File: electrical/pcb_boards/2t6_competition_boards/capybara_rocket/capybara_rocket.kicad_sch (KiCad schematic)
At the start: 110 parts, among them J1 3.6V Battery, J10 Elevator, J11 SparkFun MAX-M10S, J12 Aileron 1, J13 Aileron 2, J14 Ground Camera, J15 Payload Camera, J16 DC Motor, J2 1.2V Battery, J3 3.6V Switch, J4 1.2V Switch, J5 LED, J6 NC, J7 CC, J8 VL53L1-SATEL, J9 Egg, Q1 SI4435DDY, Q2 SI4435DDY, U1 DS1307+, U10 TPS3839, U11 MP3414, U12 SN74LVC1G04, U13 MCP1640, U14 TPS3839, U15 STM32 NUCLEO-G431KB, U16 SN74AUP1G04, U17 SparkFun XBee Explorer, U2 Adafruit BNO085, U3 TLC555, U4 EEPROM, U5 LTC3536, U6 LTC3536, U7 Adafruit BMP581, U8 DRV8212, U9 INA219, Y1 AB38T-32.768KHZ

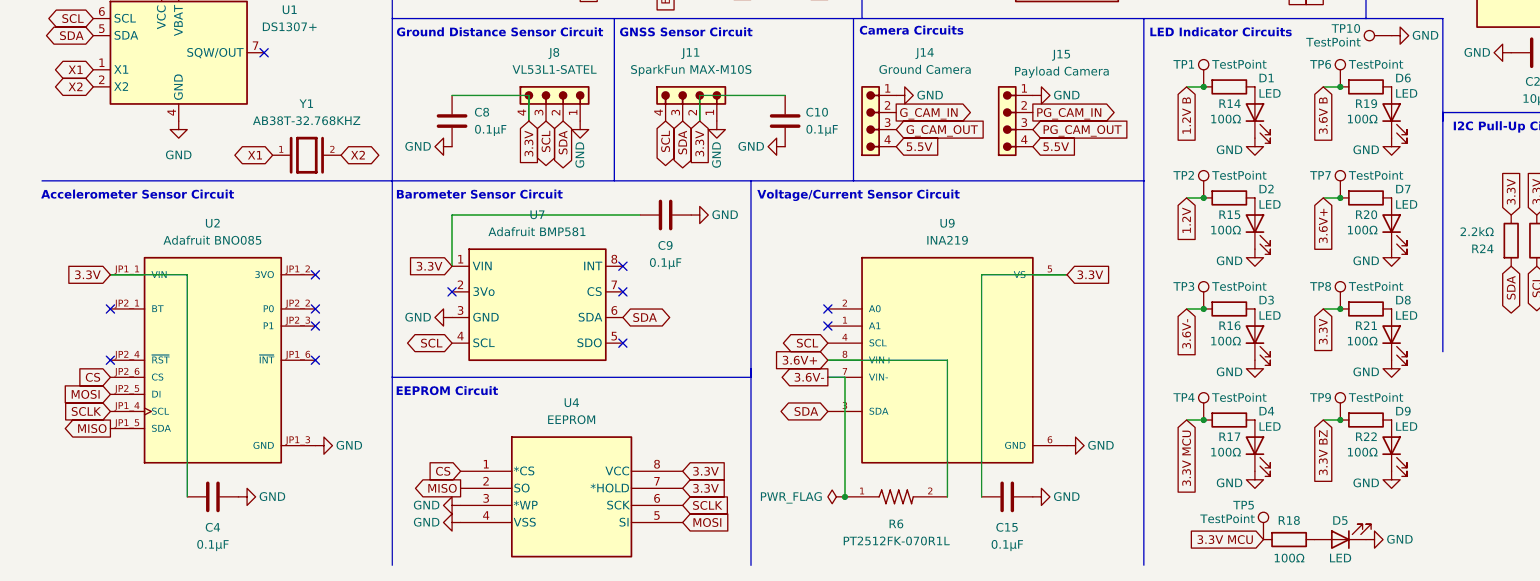
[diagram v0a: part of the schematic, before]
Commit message: New graphics and layout work
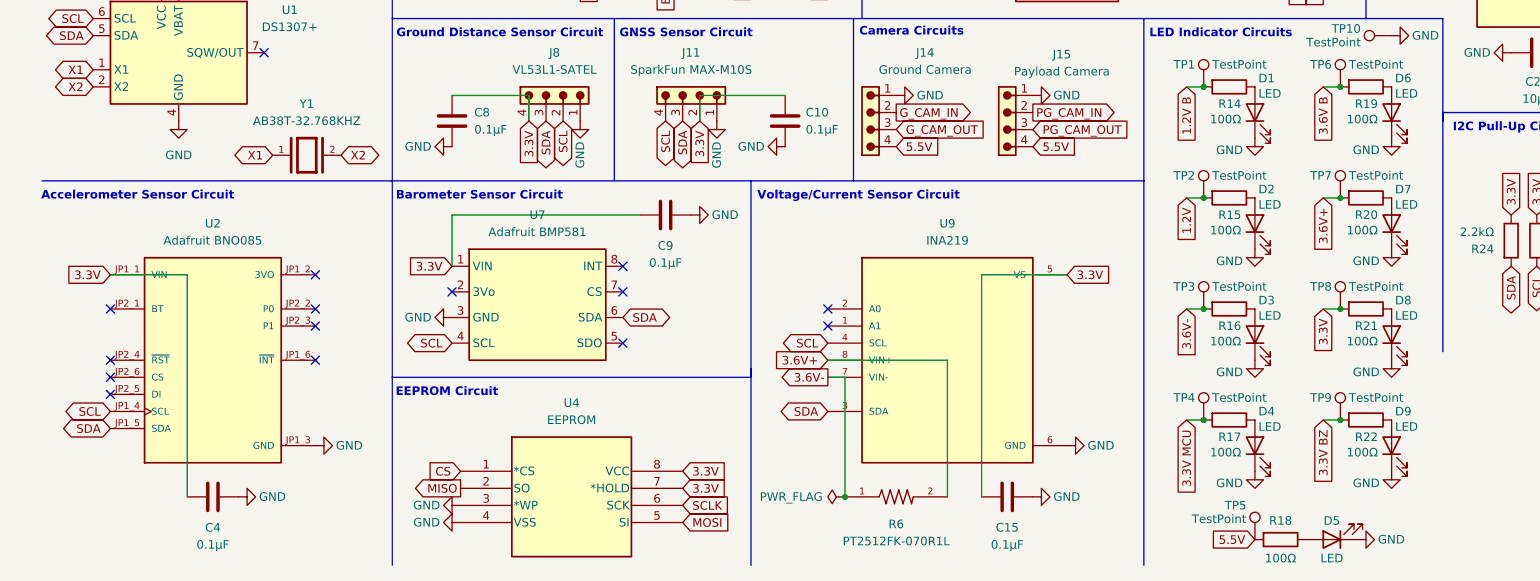
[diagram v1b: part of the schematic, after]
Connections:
- net 3.3V MCU: no longer R18.2, TP5.1
- net 5.5V: now also R18.2, TP5.1
- net CS: no longer U2.JP2_6 (CS)
- net MISO: no longer U2.JP1_5 (SDA)
- net MOSI: no longer U2.JP2_5 (DI)
- net SCL: now also J8.2, U2.JP1_4 (SCL); no longer J8.3
- net SCLK: no longer U2.JP1_4 (SCL)
- net SDA: now also J8.3, U2.JP1_5 (SDA); no longer J8.2
- no-connect marks 62 -> 64
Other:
- moved on the sheet: D5, R18, TP5
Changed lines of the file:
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@@
 	)
 	(no_connect
+		(at 22.86 171.45)
+	)
+	(no_connect
 		(at 29.21 71.12)
 	)
@@
 	)
 	(no_connect
+		(at 22.86 168.91)
+	)
+	(no_connect
 		(at 99.06 152.4)
 	)
@@
 		)
 	)
-	(global_label "MOSI"
-		(shape input)
-		(at 22.86 171.45 180)
-		(fields_autoplaced yes)
-		(effects
-			(font
-				(size 1.27 1.27)
-			)
-			(justify right)
-		)
-		(property "Intersheetrefs" "${INTERSHEET_REFS}"
-			(at 15.2786 171.45 0)
-			(effects
-				(font
-					(size 1.27 1.27)
-				)
-				(justify right)
-				(hide yes)
-			)
-		)
-	)
 	(global_label "SDA"
 		(shape bidirectional)
@@
 		)
 	)
-	(global_label "3.3V MCU"
+	(global_label "5.5V"
 		(shape input)
-		(at 194.31 193.04 180)
+		(at 193.04 193.04 180)
 		(fields_autoplaced yes)
 		(effects
@@
 		)
 		(property "Intersheetrefs" "${INTERSHEET_REFS}"
-			(at 182.1929 193.04 0)
+			(at 185.9424 193.04 0)
 			(effects
 				(font
@@
 		)
 	)
+	(global_label "SCL"
+		(shape bidirectional)
+		(at 90.17 130.81 270)
+		(fields_autoplaced yes)
+		(effects
+			(font
+				(size 1.27 1.27)
+			)
+			(justify right)
+		)
+		(property "Intersheetrefs" "${INTERSHEET_REFS}"
+			(at 90.17 138.4141 90)
+			(effects
+				(font
+					(size 1.27 1.27)
+				)
+				(justify right)
+				(hide yes)
+			)
+		)
+	)
 	(global_label "SDA"
 		(shape bidirectional)
@@
 		)
 	)
-	(global_label "SDA"
-		(shape bidirectional)
-		(at 90.17 130.81 270)
-		(fields_autoplaced yes)
-		(effects
-			(font
-				(size 1.27 1.27)
-			)
-			(justify right)
-		)
-		(property "Intersheetrefs" "${INTERSHEET_REFS}"
-			(at 90.17 138.4746 90)
-			(effects
-				(font
-					(size 1.27 1.27)
-				)
-				(justify right)
-				(hide yes)
-			)
-		)
-	)
 	(global_label "NC_REL"
 		(shape output)
@@
 		)
 	)
-	(global_label "CS"
-		(shape input)
-		(at 22.86 168.91 180)
-		(fields_autoplaced yes)
-		(effects
-			(font
-				(size 1.27 1.27)
-			)
-			(justify right)
-		)
-		(property "Intersheetrefs" "${INTERSHEET_REFS}"
-			(at 17.3953 168.91 0)
-			(effects
-				(font
-					(size 1.27 1.27)
-				)
-				(justify right)
-				(hide yes)
-			)
-		)
-	)
 	(global_label "AILERON"
 		(shape input)
@@
 		)
 	)
-	(global_label "MISO"
-		(shape output)
-		(at 22.86 176.53 180)
-		(fields_autoplaced yes)
-		(effects
-			(font
-				(size 1.27 1.27)
-			)
-			(justify right)
-		)
-		(property "Intersheetrefs" "${INTERSHEET_REFS}"
-			(at 15.2786 176.53 0)
-			(effects
-				(font
-					(size 1.27 1.27)
-				)
-				(justify right)
-				(hide yes)
-			)
-		)
-	)
 	(global_label "3.3V MCU"
 		(shape output)
@@
 		)
 	)
+	(global_label "SDA"
+		(shape bidirectional)
+		(at 22.86 176.53 180)
+		(fields_autoplaced yes)
+		(effects
+			(font
+				(size 1.27 1.27)
+			)
+			(justify right)
+		)
+		(property "Intersheetrefs" "${INTERSHEET_REFS}"
+			(at 15.1954 176.53 0)
+			(effects
+				(font
+					(size 1.27 1.27)
+				)
+				(justify right)
+				(hide yes)
+			)
+		)
+	)
 	(global_label "INV_PWM_1"
 		(shape input)
@@
 		)
 	)
+	(global_label "SCL"
+		(shape bidirectional)
+		(at 22.86 173.99 180)
+		(fields_autoplaced yes)
+		(effects
+			(font
+				(size 1.27 1.27)
+			)
+			(justify right)
+		)
+		(property "Intersheetrefs" "${INTERSHEET_REFS}"
+			(at 15.2559 173.99 0)
+			(effects
+				(font
+					(size 1.27 1.27)
+				)
+				(justify right)
+				(hide yes)
+			)
+		)
+	)
 	(global_label "DC_PWM_1"
 		(shape input)
@@
 		)
 	)
-	(global_label "SCLK"
-		(shape input)
-		(at 22.86 173.99 180)
+	(global_label "SDA"
+		(shape bidirectional)
+		(at 87.63 130.81 270)
 		(fields_autoplaced yes)
 		(effects
@@
 		)
 		(property "Intersheetrefs" "${INTERSHEET_REFS}"
-			(at 15.0972 173.99 0)
+			(at 87.63 138.4746 90)
 			(effects
 				(font
@@
 		)
 	)
-	(global_label "SCL"
-		(shape bidirectional)
-		(at 87.63 130.81 270)
-		(fields_autoplaced yes)
-		(effects
-			(font
-				(size 1.27 1.27)
-			)
-			(justify right)
-		)
-		(property "Intersheetrefs" "${INTERSHEET_REFS}"
-			(at 87.63 138.4141 90)
-			(effects
-				(font
-					(size 1.27 1.27)
-				)
-				(justify right)
-				(hide yes)
-			)
-		)
-	)
 	(global_label "G_CAM_OUT"
 		(shape input)
@@
 	(symbol
 		(lib_id "Device:R")
-		(at 198.12 193.04 270)
+		(at 196.85 193.04 270)
 		(unit 1)
 		(exclude_from_sim no)
@@
 		(dnp no)
 		(property "Reference" "R18"
-			(at 198.12 190.246 90)
+			(at 196.85 190.246 90)
 			(effects
 				(font
@@
 		)
 		(property "Value" "100Ω"
-			(at 198.12 195.834 90)
+			(at 196.85 195.834 90)
 			(effects
 				(font
@@
 		)
 		(property "Footprint" "Resistor_SMD:R_0603_1608Metric_Pad0.98x0.95mm_HandSolder"
-			(at 198.12 191.262 90)
+			(at 196.85 191.262 90)
 			(effects
 				(font
@@
 		)
 		(property "Datasheet" "~"
-			(at 198.12 193.04 0)
+			(at 196.85 193.04 0)
 			(effects
 				(font
@@
 		)
 		(property "Description" "Resistor"
-			(at 198.12 193.04 0)
+			(at 196.85 193.04 0)
 			(effects
 				(font
@@
 	(symbol
 		(lib_id "power:GND")
-		(at 209.55 193.04 90)
+		(at 208.28 193.04 90)
 		(unit 1)
 		(exclude_from_sim no)
@@
 		(dnp no)
 		(property "Reference" "#PWR053"
-			(at 215.9 193.04 0)
+			(at 214.63 193.04 0)
 			(effects
 				(font
@@
 		)
 		(property "Value" "GND"
-			(at 212.598 193.04 90)
+			(at 211.328 193.04 90)
 			(effects
 				(font
@@
 		)
 		(property "Footprint" ""
-			(at 209.55 193.04 0)
+			(at 208.28 193.04 0)
 			(effects
 				(font
@@
 		)
 		(property "Datasheet" ""
-			(at 209.55 193.04 0)
+			(at 208.28 193.04 0)
 			(effects
 				(font
@@
 		)
 		(property "Description" "Power symbol creates a global label with name \"GND\" , ground"
-			(at 209.55 193.04 0)
+			(at 208.28 193.04 0)
 			(effects
 				(font
@@
 	(symbol
 		(lib_id "Device:LED")
-		(at 205.74 193.04 180)
+		(at 204.47 193.04 180)
 		(unit 1)
 		(exclude_from_sim no)
@@
 		(dnp no)
 		(property "Reference" "D5"
-			(at 205.74 190.246 0)
+			(at 204.47 190.246 0)
 			(effects
 				(font
@@
 		)
 		(property "Value" "LED"
-			(at 205.74 195.834 0)
+			(at 204.47 195.834 0)
 			(effects
 				(font
@@
 		)
 		(property "Footprint" "DigiKey:WL-SMCW_0603"
-			(at 205.74 193.04 0)
+			(at 204.47 193.04 0)
 			(effects
 				(font
@@
 		)
 		(property "Datasheet" "~"
-			(at 205.74 193.04 0)
+			(at 204.47 193.04 0)
 			(effects
 				(font
@@
 		)
 		(property "Description" "Light emitting diode"
-			(at 205.74 193.04 0)
+			(at 204.47 193.04 0)
 			(effects
 				(font
@@
 		)
 		(property "Sim.Pins" "1=K 2=A"
-			(at 205.74 193.04 0)
+			(at 204.47 193.04 0)
 			(effects
 				(font
@@
 	(symbol
 		(lib_id "Connector:TestPoint")
-		(at 194.31 193.04 0)
+		(at 193.04 193.04 0)
 		(unit 1)
 		(exclude_from_sim no)
@@
 		(dnp no)
 		(property "Reference" "TP5"
-			(at 193.04 187.96 0)
+			(at 191.77 187.96 0)
 			(effects
 				(font
@@
 		)
 		(property "Value" "TestPoint"
-			(at 193.04 189.992 0)
+			(at 191.77 189.992 0)
 			(effects
 				(font
@@
 		)
 		(property "Footprint" "TestPoint:TestPoint_THTPad_2.0x2.0mm_Drill1.0mm"
-			(at 199.39 193.04 0)
+			(at 198.12 193.04 0)
 			(effects
 				(font
@@
 		)
 		(property "Datasheet" "~"
-			(at 199.39 193.04 0)
+			(at 198.12 193.04 0)
 			(effects
 				(font
@@
 		)
 		(property "Description" "test point"
-			(at 194.31 193.04 0)
+			(at 193.04 193.04 0)
 			(effects
 				(font
